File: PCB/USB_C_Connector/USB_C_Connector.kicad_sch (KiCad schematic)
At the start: 10 parts, among them J1 USB_C_Receptacle_USB2.0_16P, J2 Conn_01x20, J3 Conn_01x20, J4 SSD1306, SW1 SW_Push, SW2 SW_Push, U2 USBLC6-2SC6

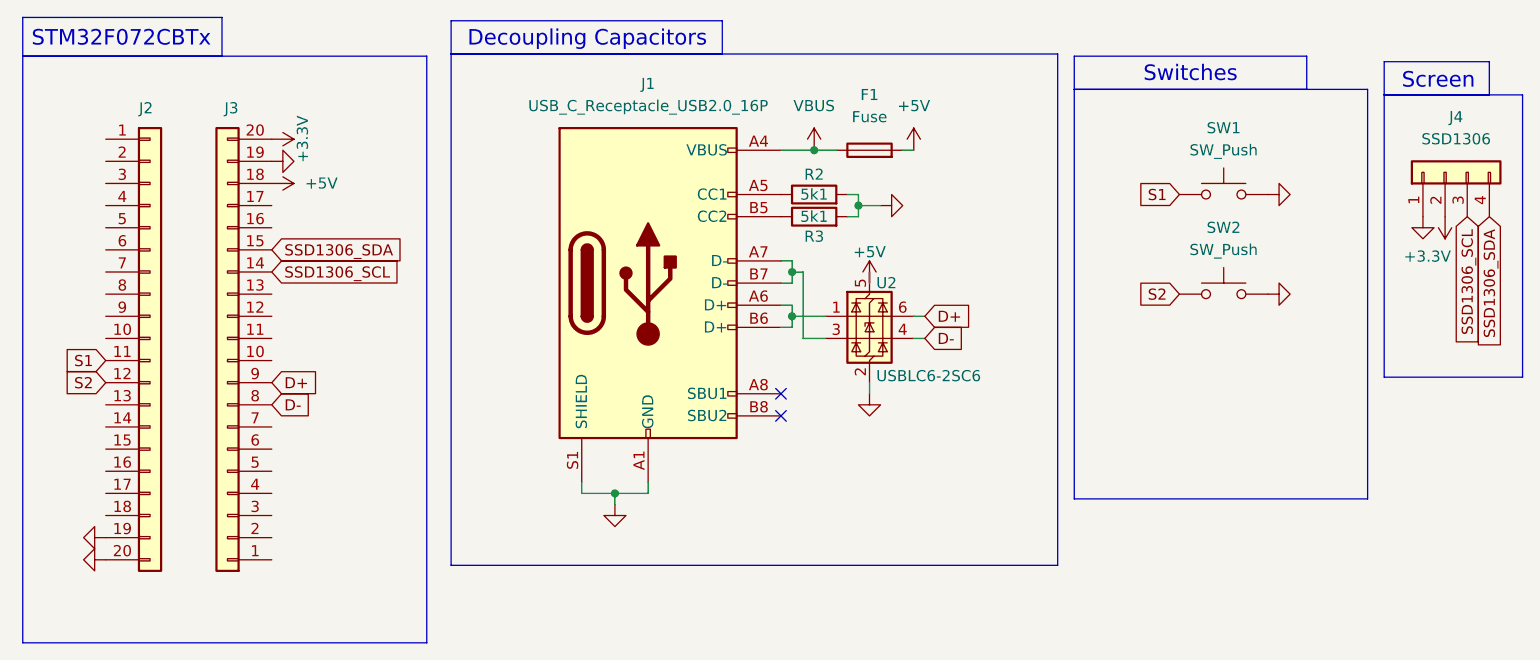
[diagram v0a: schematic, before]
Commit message: Add many things
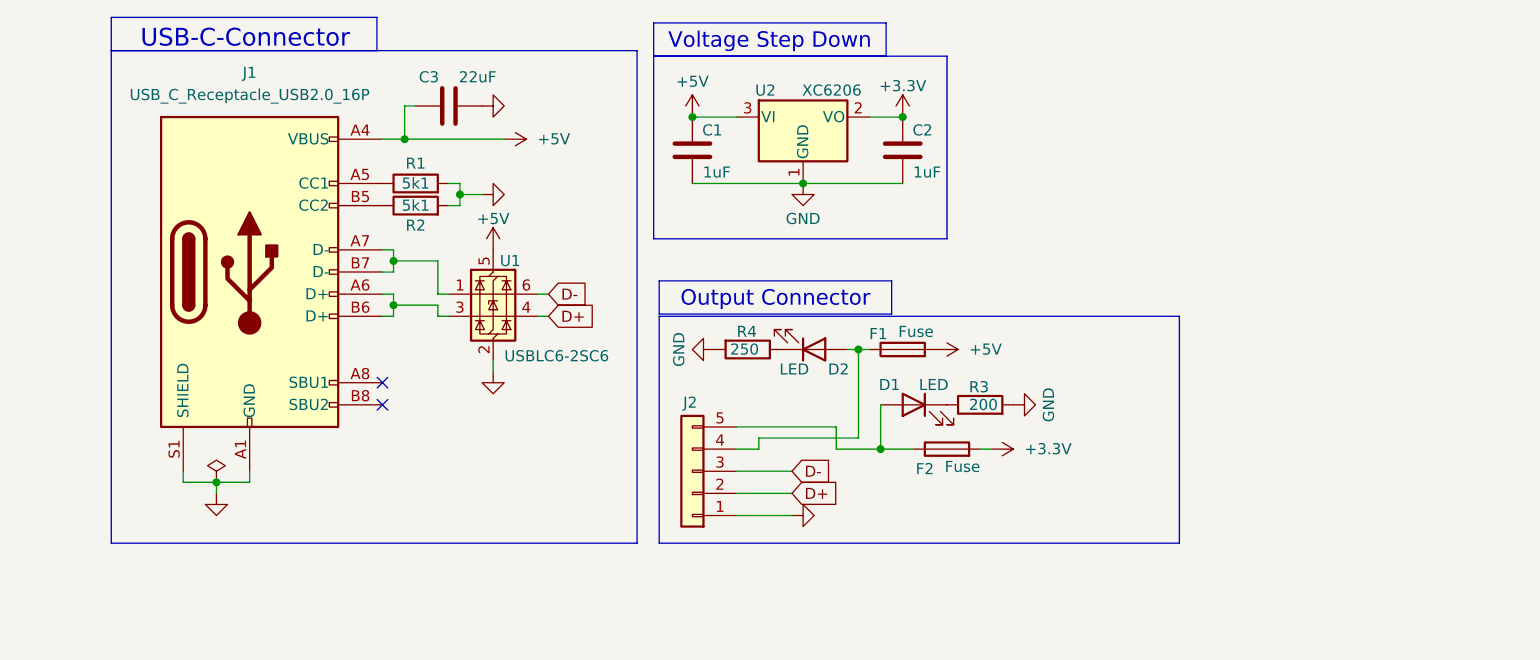
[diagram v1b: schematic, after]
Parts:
- removed J2, J3: Conn_01x20, symbol Connector_Generic:Conn_01x20
- removed J4: SSD1306, symbol Connector_Generic:Conn_01x04
- removed SW1, SW2: SW_Push, symbol Switch:SW_Push
- removed U2: USBLC6-2SC6, Package_TO_SOT_SMD:SOT-23-6, symbol Power_Protection:USBLC6-2SC6
- added C1, C2: 1uF, Capacitor_SMD:C_0603_1608Metric_Pad1.08x0.95mm_HandSolder, symbol Device:C
- added C3: 22uF, Capacitor_SMD:C_0603_1608Metric_Pad1.08x0.95mm_HandSolder, symbol Device:C
- added D1, D2: LED, LED_SMD:LED_0805_2012Metric, symbol Device:LED
- added F2: Fuse, Fuse:Fuse_0603_1608Metric_Pad1.05x0.95mm_HandSolder, symbol Device:Fuse
- added J2: Conn_01x05, Connector_PinHeader_2.54mm:PinHeader_1x05_P2.54mm_Vertical, symbol Connector_Generic:Conn_01x05
- added R1: 5k1, Resistor_SMD:R_0603_1608Metric_Pad0.98x0.95mm_HandSolder, symbol Device:R
- added R4: 250, Resistor_SMD:R_0603_1608Metric_Pad0.98x0.95mm_HandSolder, symbol Device:R
- added U1: USBLC6-2SC6, Package_TO_SOT_SMD:SOT-23-6, symbol Power_Protection:USBLC6-2SC6
- added U2: XC6206, Package_TO_SOT_SMD:SOT-23-3, symbol Regulator_Linear:XC6206PxxxMR
- F1: footprint (none) -> Fuse:Fuse_0603_1608Metric_Pad1.05x0.95mm_HandSolder
- J1: footprint (none) -> Connector_USB:USB_C_Receptacle_HRO_TYPE-C-31-M-12
- R2: footprint (none) -> Resistor_SMD:R_0603_1608Metric_Pad0.98x0.95mm_HandSolder
- R3: value 5k1 -> 200; footprint (none) -> Resistor_SMD:R_0603_1608Metric_Pad0.98x0.95mm_HandSolder
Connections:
- net +3.3V: now also C2.1, F2.2, U2.2 (VO)
- net +5V: now also J1.A4 (VBUS), J1.A9 (VBUS), J1.B4 (VBUS), J1.B9 (VBUS), C1.1, C3.1, U1.5 (VBUS), U2.3 (VI)
- net D+: now also J2.2 (Pin_2), U1.4 (I/O2)
- net D-: now also J2.3 (Pin_3), U1.6 (I/O1)
- net GND: now also C1.2, C2.2, C3.2, J2.1 (Pin_1), R1.2, R4.2, U1.2 (GND), U2.1 (GND)
- net at R3.1: now also D1.1 (K); no longer J1.B5 (CC2)
- net at J1.A6 (D+), J1.B6 (D+): now also U1.3 (I/O2)
- net at J1.A7 (D-), J1.B7 (D-): now also U1.1 (I/O1)
- net at J1.A5 (CC1): now also R1.1; no longer R2.1
- removed net VBUS: F1.1, J1.A4 (VBUS), J1.A9 (VBUS), J1.B4 (VBUS), J1.B9 (VBUS)
- new net: D1.2 (A), F2.1, J2.5 (Pin_5)
- new net: D2.1 (K), R4.1
- new net: D2.2 (A), F1.1, J2.4 (Pin_4)
- new net: J1.B5 (CC2), R2.1
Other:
- note added: "Output Connector"
- note added: "USB-C-Connector"
- note added: "Voltage Step Down"
- note removed: "Decoupling Capacitors"
- note removed: "STM32F072CBTx"
- note removed: "Screen"
- note removed: "Switches"
